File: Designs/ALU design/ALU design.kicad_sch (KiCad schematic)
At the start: 41 parts, among them U1 74LS86, U10 74LS08, U11 74LS125, U12 74LS125, U13 74LS32, U14 74LS138, U15 74LS125, U2 74LS86, U3 74LS173, U4 74LS83, U5 74LS173, U6 74LS173, U7 74LS173, U8 74LS125, U9 74LS86

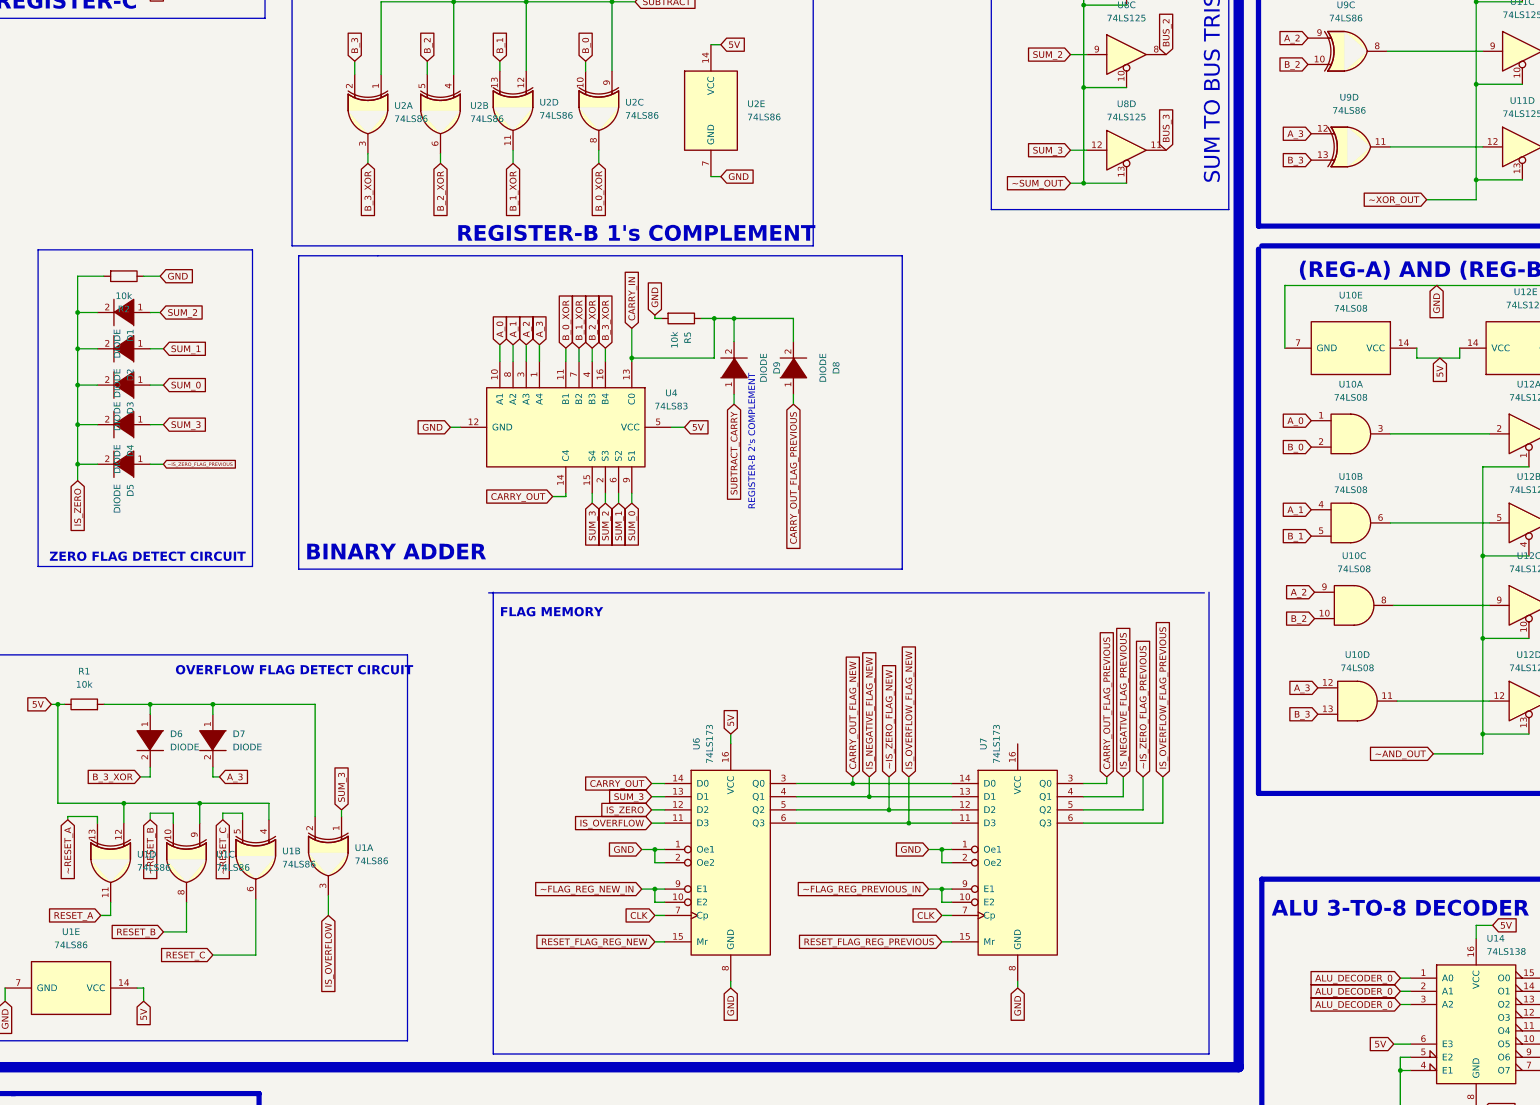
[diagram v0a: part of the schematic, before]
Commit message: Update ALU design.kicad_sch
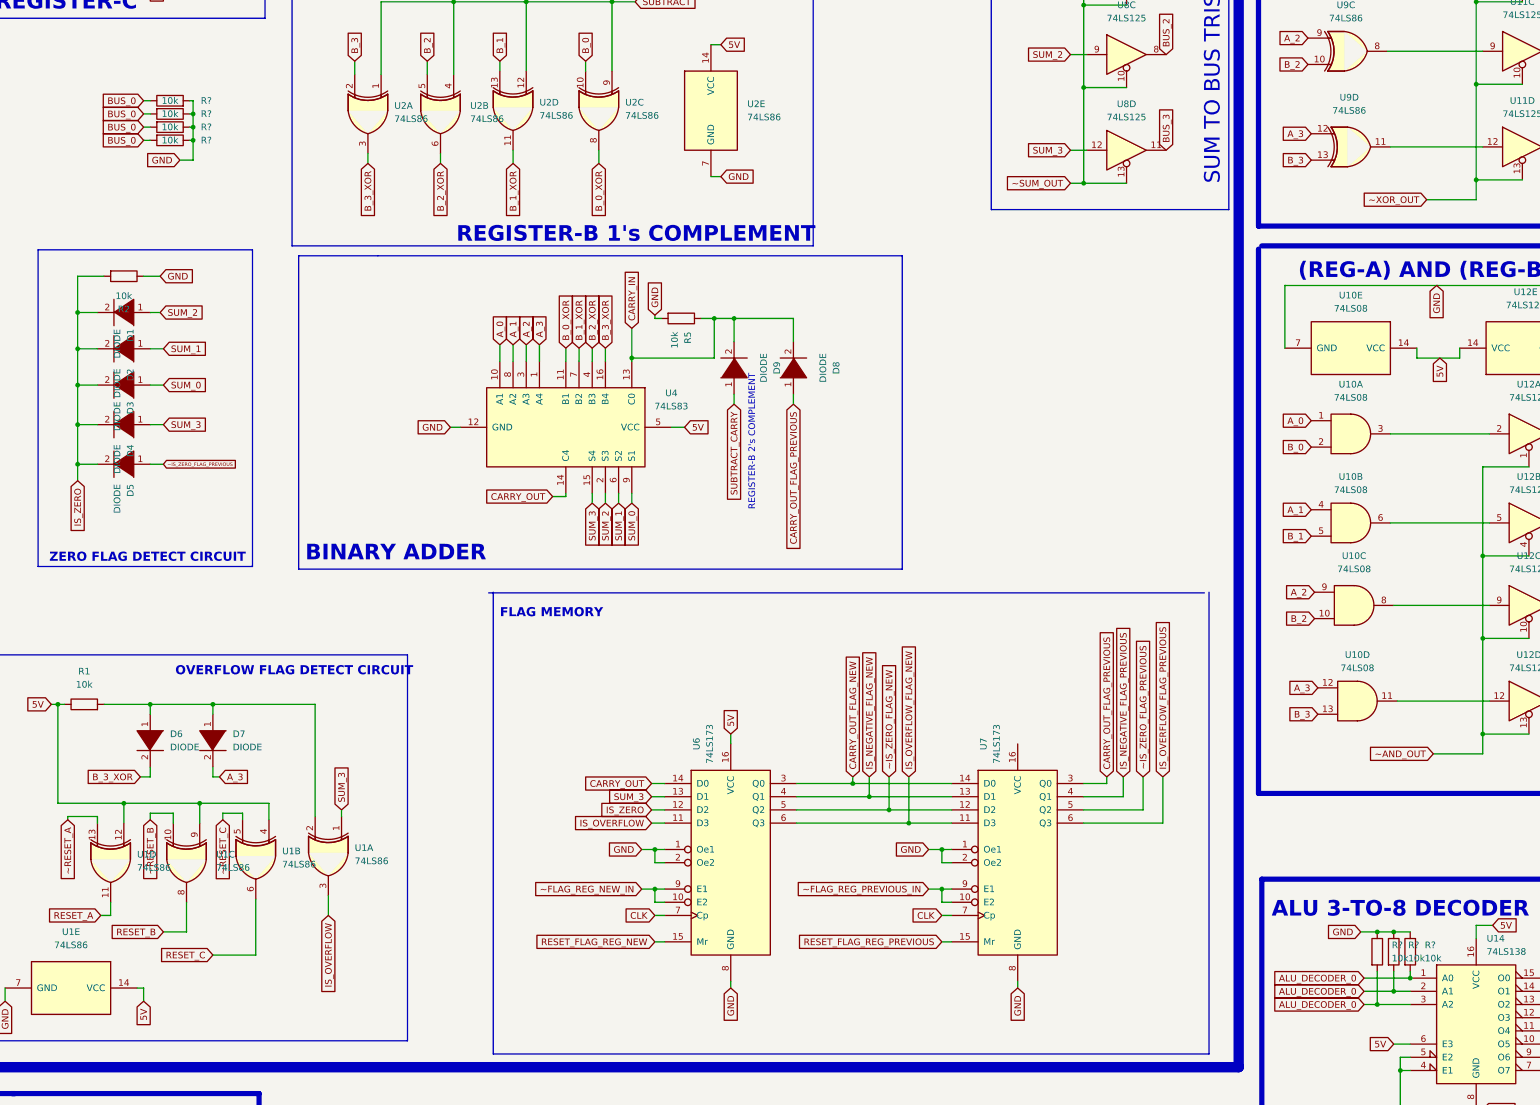
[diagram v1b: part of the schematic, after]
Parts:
- added R? (x7): 10k, symbol Device:R
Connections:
- net ALU_DECODER_0: now also R?.2, R?.2, R?.2
- net BUS_0: now also R?.1, R?.2, R?.2, R?.2
- net GND: now also R?.1, R?.1, R?.1, R?.1, R?.1, R?.1, R?.2
